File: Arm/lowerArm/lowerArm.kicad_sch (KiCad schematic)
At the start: 4 parts, among them J1 Screw_Terminal_01x12, J2 Screw_Terminal_01x12, U1 LM1084-5.0

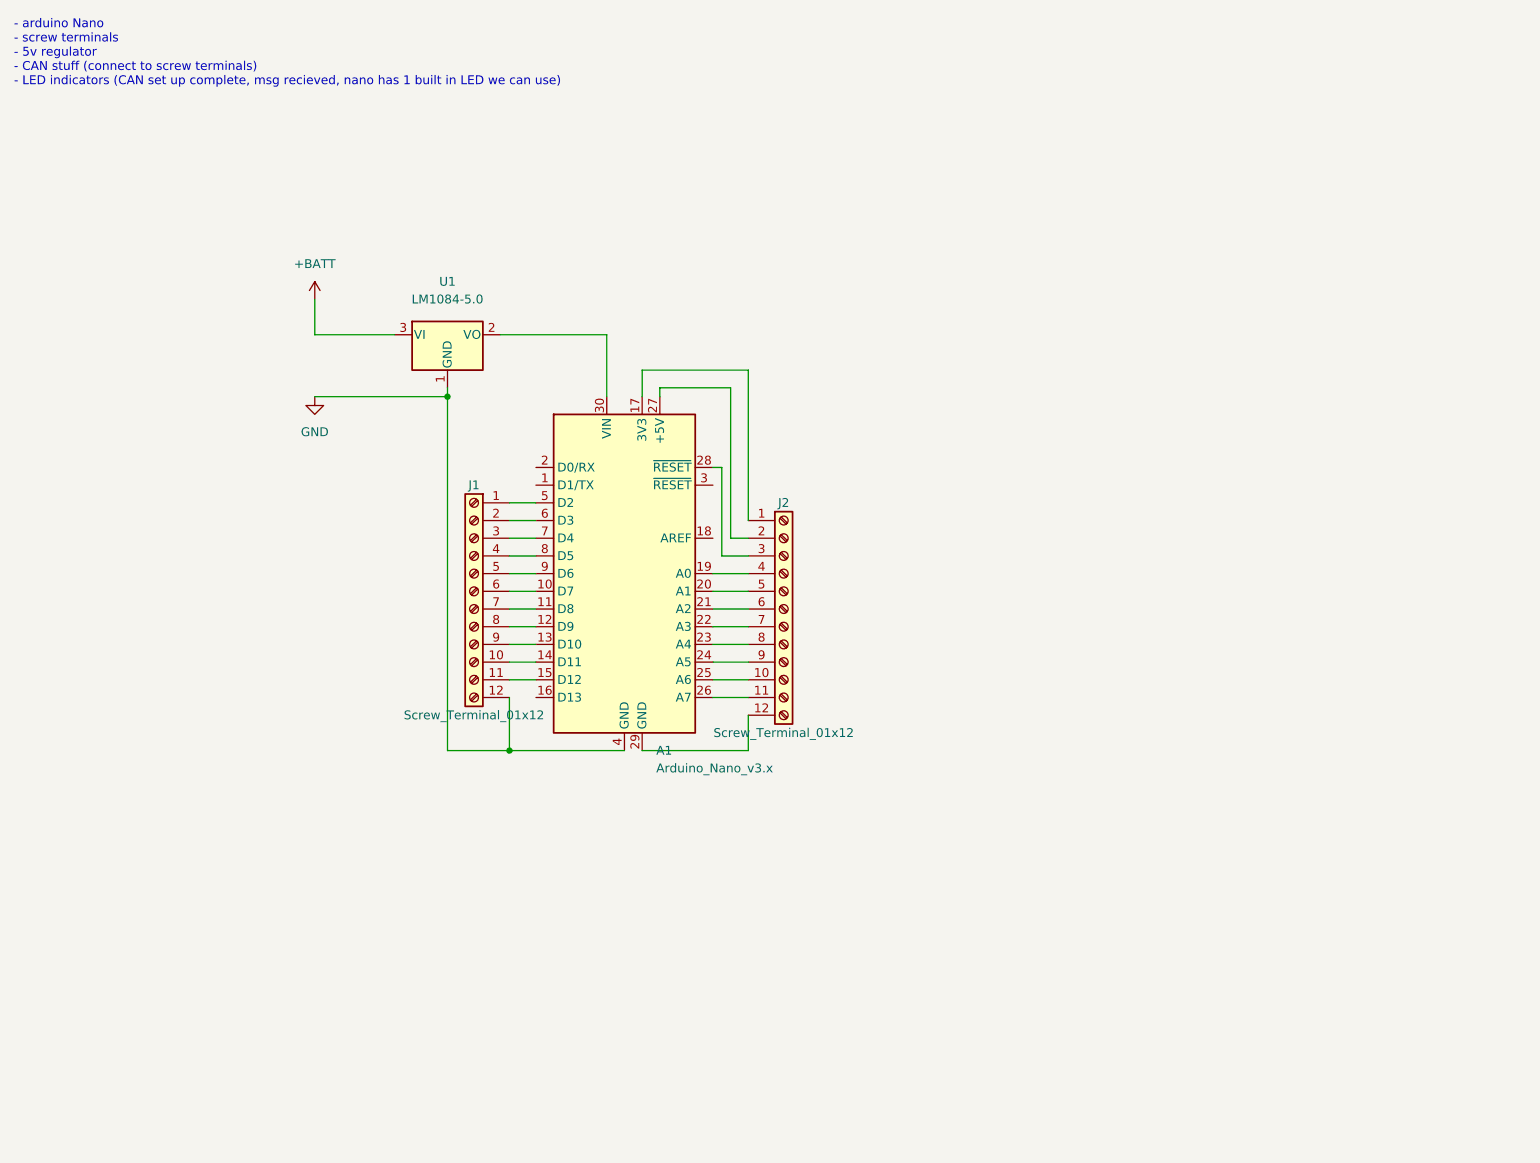
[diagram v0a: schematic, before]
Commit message: updated Arm arduino code, manual_operate, and PCBs
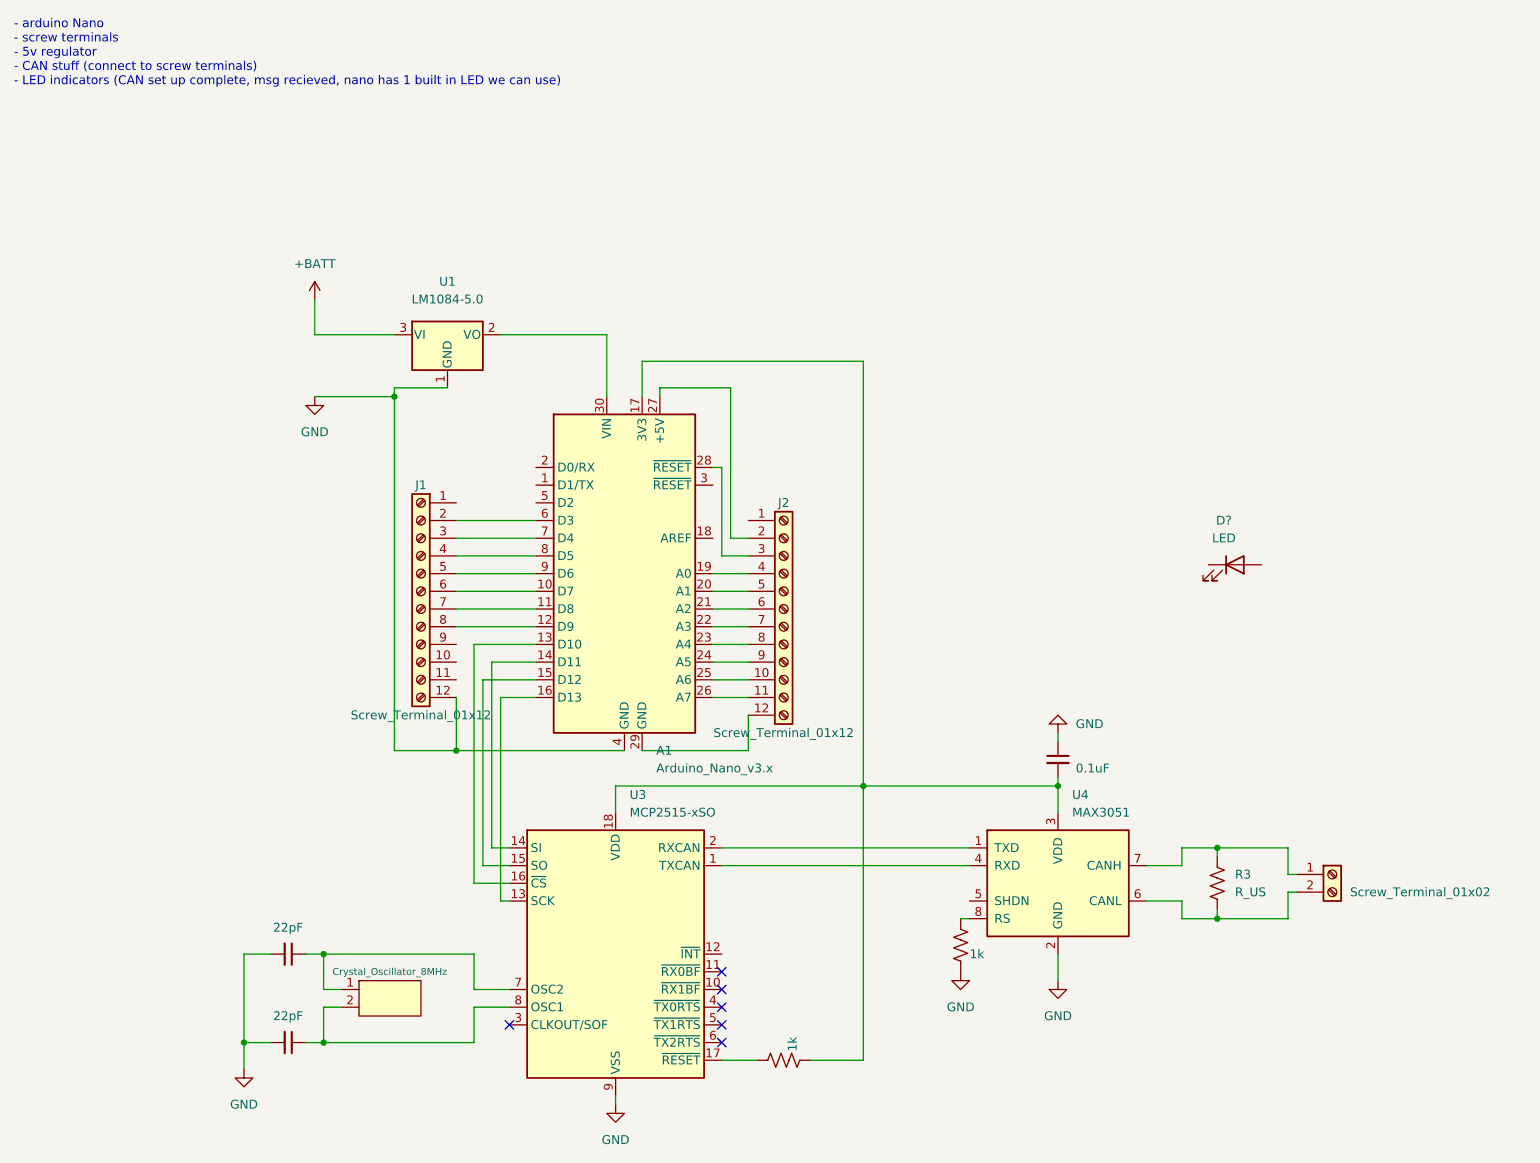
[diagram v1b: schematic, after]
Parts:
- added C1: 0.1uF, Capacitor_SMD:C_0805_2012Metric, symbol Device:C_Small
- added C2, C3: 22pF, Capacitor_SMD:C_0805_2012Metric, symbol Device:C_Small
- added D?: LED, symbol Device:LED
- added J3: Screw_Terminal_01x02, TerminalBlock_4Ucon:TerminalBlock_4Ucon_1x02_P3.50mm_Horizontal, symbol Connector:Screw_Terminal_01x02
- added R1, R2: 1k, Resistor_SMD:R_0805_2012Metric, symbol Device:R_US
- added R3: R_US, Resistor_SMD:R_0805_2012Metric, symbol Device:R_US
- added U2: Crystal_Oscillator_8MHz, LFXTAL:LFXTAL057135Bulk, symbol customSymbols:Crystal_Oscillator_8MHz
- added U3: MCP2515-xSO, MCP2515_SMD:SOIC127P1030X265-18N, symbol Interface_CAN_LIN:MCP2515-xSO
- added U4: MAX3051, MAX3051:SOIC127P600X175-8N, symbol Interface_UART:MAX3051
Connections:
- net GND: now also C1.1, C2.2, C3.2, R1.2, U3.9 (VSS), U4.2 (GND)
- net at J2.1 (Pin_1): no longer A1.17 (3V3)
- net at J1.1 (Pin_1): no longer A1.5 (D2)
- net at J1.10 (Pin_10): no longer A1.14 (D11)
- net at J1.11 (Pin_11): no longer A1.15 (D12)
- net at J1.9 (Pin_9): no longer A1.13 (D10)
- net at A1.16 (D13): now also U3.13 (SCK)
- new net: R2.1, U3.17 (~{RESET})
- new net: A1.17 (3V3), C1.2, R2.2, U3.18 (VDD), U4.3 (VDD)
- new net: C3.1, U2.2, U3.8 (OSC1)
- new net: C2.1, U2.1, U3.7 (OSC2)
- new net: A1.13 (D10), U3.16 (~{CS})
- new net: A1.14 (D11), U3.14 (SI)
- new net: A1.15 (D12), U3.15 (SO)
- new net: U3.2 (RXCAN), U4.1 (TXD)
- new net: U3.1 (TXCAN), U4.4 (RXD)
- new net: J3.2 (Pin_2), R3.2, U4.6 (CANL)
- new net: J3.1 (Pin_1), R3.1, U4.7 (CANH)
- new net: R1.1, U4.8 (RS)
- no-connect marks 0 -> 6
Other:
- moved on the sheet: J1
